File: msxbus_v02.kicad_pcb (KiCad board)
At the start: 2 copper layers, 4 parts, among them J1 RPi_GPIO, P1 MSX_SLOT, P2 MSX_SLOT, U1 CPLD

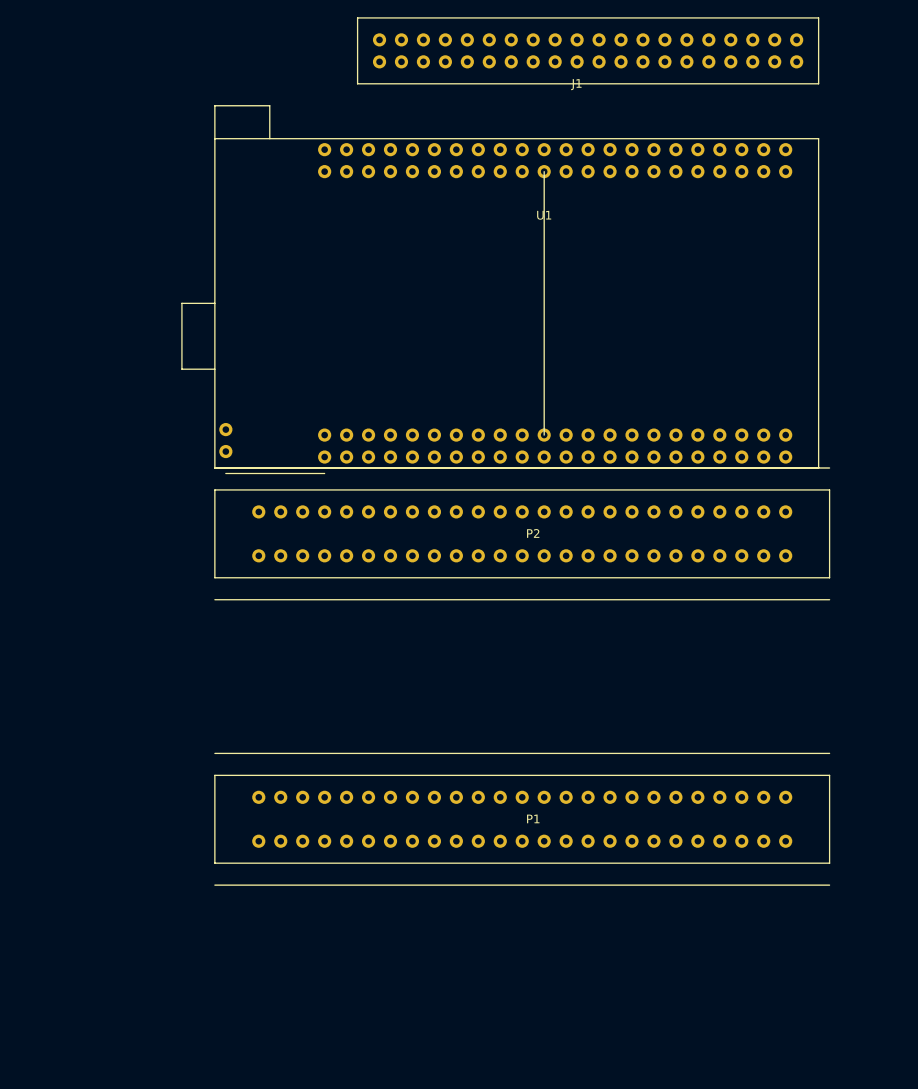
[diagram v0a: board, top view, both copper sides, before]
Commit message: PCB update
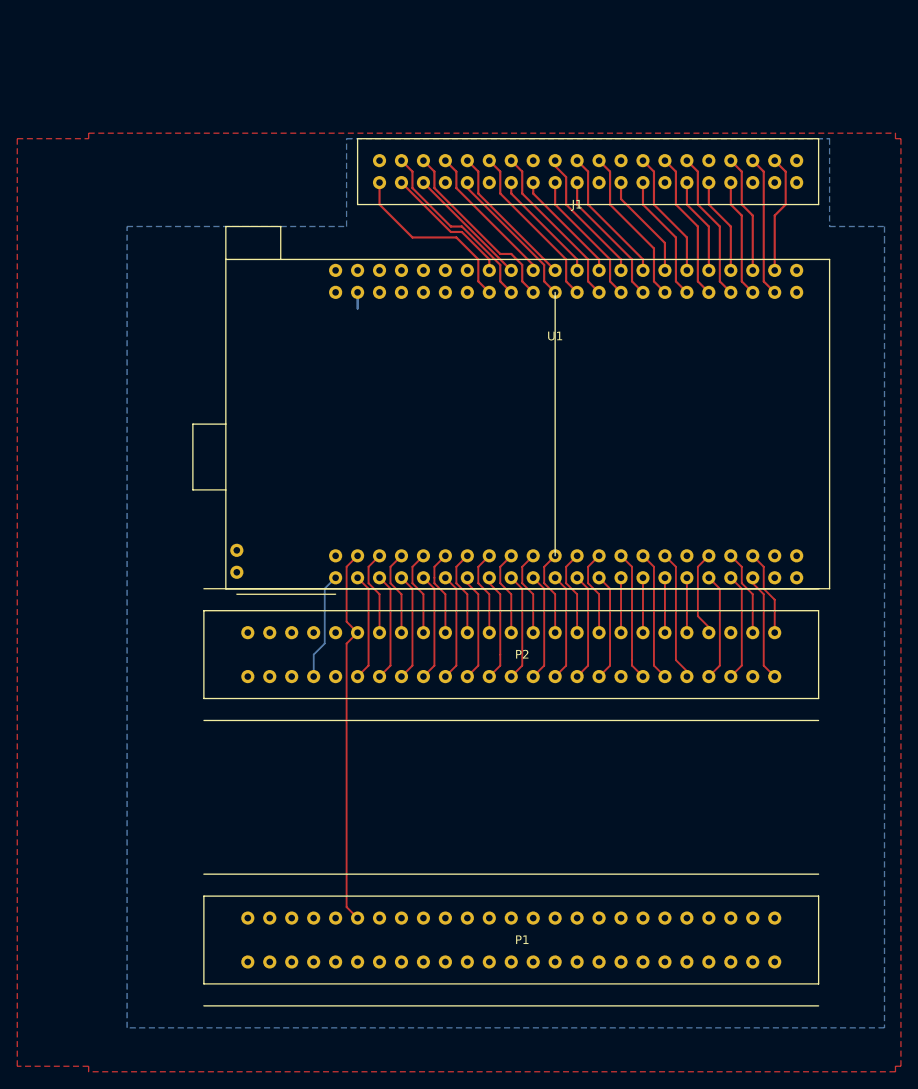
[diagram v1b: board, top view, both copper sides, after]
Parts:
- moved P2 14.0 mm to (143.5, 102.9)
- moved U1 14.0 mm to (147.3, 78.7)
- moved P1 14.0 mm to (143.5, 135.9)
- moved J1 14.0 mm to (151.1, 47.0)
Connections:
- P1 pad 44: /SW1 -> /SWOUT
- P1 pad 46: /SW2 -> /SW1
- P2 pad 4: /SLTSL1 -> /SLTSL2
- P2 pad 44: /SW1 -> /SWOUT
- U1 pad 1: Net-(U1-Pad1) -> /GND
- U1 pad 10: /RG15 -> /RG27
- U1 pad 11: /RG17 -> /RG22
- U1 pad 12: /RG18 -> /RG23
- U1 pad 13: /RG27 -> /RG24
- U1 pad 14: /RG22 -> /RG10
- U1 pad 15: /RG23 -> /RG09
- U1 pad 16: /RG24 -> /RG25
- U1 pad 17: /RG10 -> /RG11
- U1 pad 18: /RG09 -> /RG08
- U1 pad 19: /RG25 -> /RG07
- U1 pad 2: Net-(U1-Pad2) -> /GND
- U1 pad 20: /RG11 -> /RG00
- U1 pad 21: /RG08 -> /RG01
- U1 pad 22: /RG07 -> /RG05
- U1 pad 23: /RG00 -> /RG06
- U1 pad 24: /RG01 -> /RG12
- U1 pad 25: /RG05 -> /RG13
- U1 pad 26: /RG06 -> /RG19
- U1 pad 27: /RG12 -> /RG16
- U1 pad 28: /RG13 -> /RG26
- U1 pad 29: /RG19 -> /RG20
- U1 pad 3: Net-(U1-Pad3) -> /RG02
- U1 pad 30: /RG16 -> /RG21
- U1 pad 31: /RG26 -> Net-(U1-Pad31)
- U1 pad 32: /RG20 -> Net-(U1-Pad32)
- U1 pad 33: /RG21 -> Net-(U1-Pad33)
- U1 pad 34: /RG04 -> Net-(U1-Pad34)
- U1 pad 4: Net-(U1-Pad4) -> /RG03
- U1 pad 41: Net-(U1-Pad41) -> /SW2
- U1 pad 42: Net-(U1-Pad42) -> /SW1
- U1 pad 44: Net-(U1-Pad44) -> /GND
- U1 pad 45: /SW1 -> /SWOUT
- U1 pad 46: /SW2 -> /CLOCK
- U1 pad 47: /SWOUT -> /D6
- U1 pad 48: /CLOCK -> /D7
- U1 pad 49: /D6 -> /D4
- U1 pad 5: Net-(U1-Pad5) -> /RG04
- U1 pad 50: /D7 -> /D5
- U1 pad 6: /RG02 -> /RG14
- U1 pad 7: /RG03 -> /RG15
- U1 pad 8: /RG04 -> /RG17
- U1 pad 9: /RG14 -> /RG18
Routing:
- net /D7: track 0.00 -> 44.0 mm
- net /RG26: track 0.00 -> 21.2 mm
- net /RG19: track 0.00 -> 21.2 mm
- net /RG21: track 0.00 -> 20.9 mm
- net /RG05: track 0.00 -> 19.4 mm
- net /RG00: track 0.00 -> 19.4 mm
- net /RG10: track 0.00 -> 18.4 mm
- net /RG27: track 0.00 -> 17.3 mm
- net /RG17: track 0.00 -> 17.3 mm
- net /RG13: track 0.00 -> 16.9 mm
- net /RG12: track 0.00 -> 16.9 mm
- net /RG06: track 0.00 -> 16.9 mm
- net /RG03: track 0.00 -> 16.3 mm
- net /RG11: track 0.00 -> 15.9 mm
- net /RG08: track 0.00 -> 15.9 mm
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- added copper zone on B.Cu, net /GND
- added copper zone on F.Cu, net /GND
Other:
- net class Default: clearance 0.2 -> 0.18; trace_width 0.25 -> 0.22
- rule trace_clearance: 0.2 -> 0.18
